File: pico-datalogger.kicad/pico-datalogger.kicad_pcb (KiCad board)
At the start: 2 copper layers, 21 x 33.8 mm, 18 parts, among them J1 JST-PH2 Bat, J2 Pico Pin 1-13, J3 Pico Pin 40-28, J4 Alt-Bat, SW1 SW_Push_SLIM, U1 SN74HC74N, U2 PCF8563T, Y1 Crystal

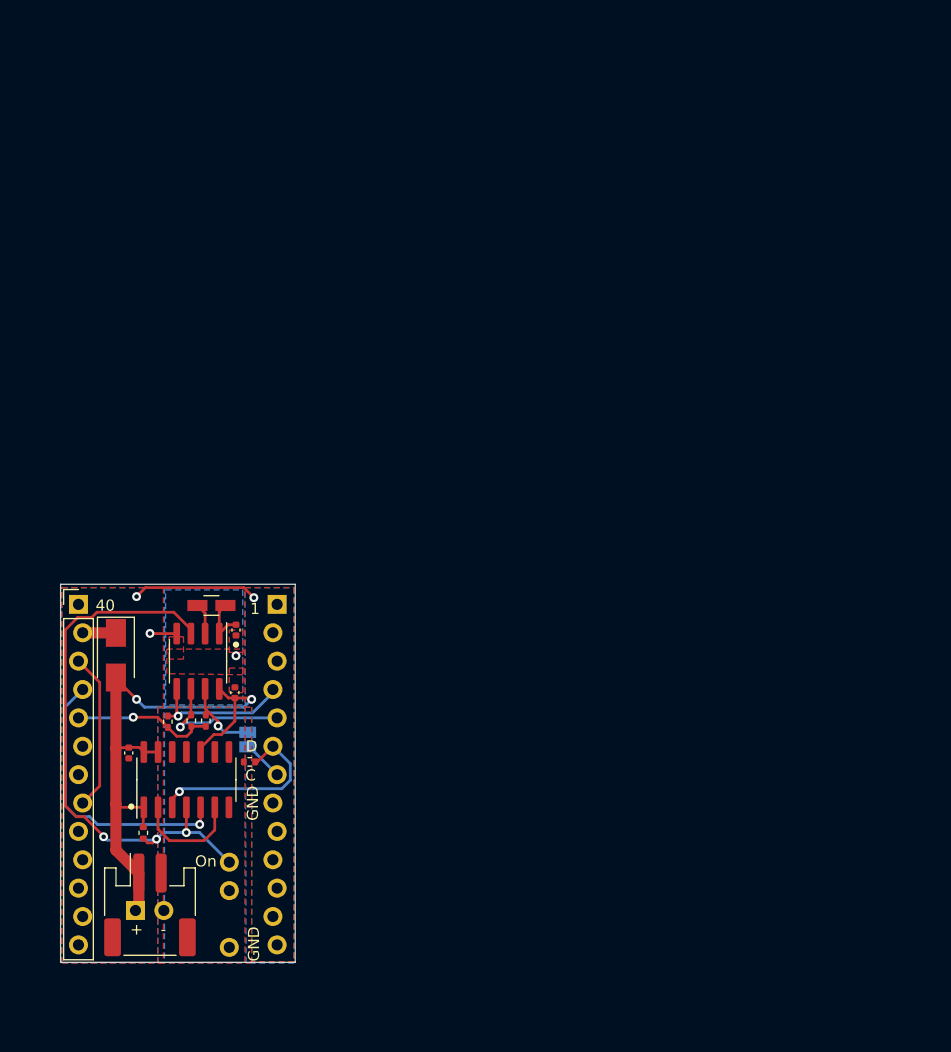
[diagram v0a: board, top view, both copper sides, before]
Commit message: Rev. 0.9: initial routing
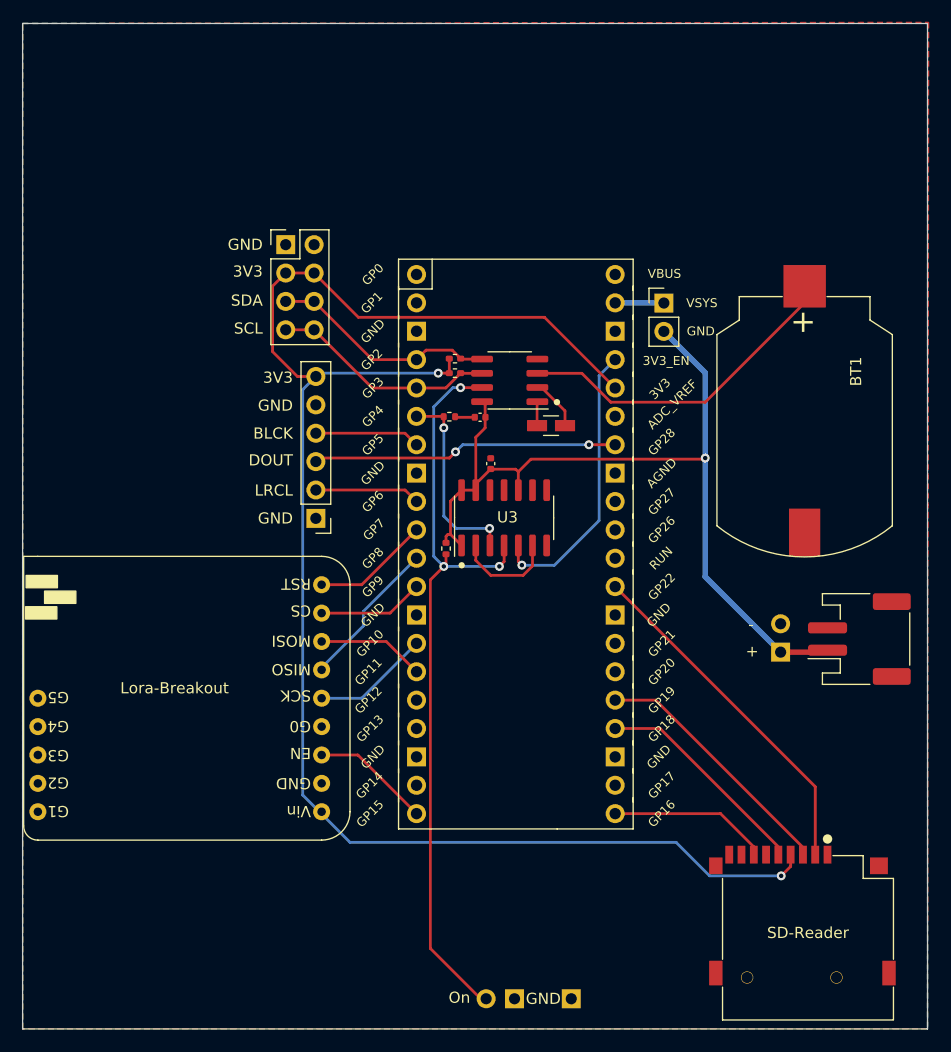
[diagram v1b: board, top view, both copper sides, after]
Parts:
- removed C3: 22pF, Capacitor_SMD:C_0402_1005Metric
- removed D1: D_Schottky, Diode_SMD:D_SMA
- removed R5: 10K, Resistor_SMD:R_0402_1005Metric
- added BT1: Coin_Cell, user:CR2032_Holder, F.Cu at (165.0, 82.5)
- added J5: Conn_I2S, Connector_PinHeader_2.54mm:PinHeader_1x06_P2.54mm_Vertical, F.Cu at (121.2, 92.3)
- added J7: Micro_SD_TF_PUSH, user:TF-Push, F.Cu at (164.8, 127.7)
- added U3: Pico, user:RPi_Pico_TH_nodbg, F.Cu at (139.2, 94.6)
- J1: value JST-PH2 Bat -> JST-PH2 VCC
- J2: value Pico Pin 1-13 -> Conn_I2C_Internal; footprint user:Connector_1x13_no_solder -> Connector_PinHeader_2.54mm:PinHeader_2x04_P2.54mm_Vertical; moved to F.Cu
- J3: value Pico Pin 40-28 -> RFM9x_Lora_Breakout; footprint user:Connector_1x13_no_solder -> user:RFM9x_Lora_Breakout
- J4: value Alt-Bat -> Alt-VCC
- JP1: value Jmp_CLKOUT -> Jumper_VSYS; footprint Jumper:SolderJumper-2_P1.3mm_Open_Pad1.0x1.5mm -> Connector_PinHeader_2.54mm:PinHeader_1x02_P2.54mm_Vertical; moved to F.Cu
- U2: value PCF8563T -> PCF8523T
- moved J1 67.8 mm to (169.9, 103.1), turned to 90 degrees
- moved J4 62.2 mm to (162.8, 104.3), turned to 0 degrees
- moved JP1 54.0 mm to (152.4, 73.0), turned to 0 degrees
- moved C1 41.5 mm to (136.9, 87.4), turned to 90 degrees
- moved R4 40.4 mm to (133.7, 79.3), turned to 0 degrees
- moved R3 40.1 mm to (133.7, 78.0), turned to 0 degrees
- moved U2 37.6 mm to (138.6, 80.0), turned to 180 degrees
- moved R2 37.2 mm to (132.9, 95.0)
- moved U1 36.9 mm to (138.1, 92.2)
- moved R1 35.7 mm to (133.2, 83.2), turned to 180 degrees
- moved Y1 34.4 mm to (142.3, 84.0), turned to 0 degrees
- moved C2 33.0 mm to (135.9, 83.2), turned to 180 degrees
- moved J2 32.2 mm to (118.5, 67.8), turned to 0 degrees
- moved SW1 31.0 mm to (144.1, 135.3), turned to 180 degrees
- moved J3 28.6 mm to (121.8, 118.6), turned to 90 degrees
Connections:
- J2 pad 1: unconnected-(J2-Pad1) -> GND
- J2 pad 2: unconnected-(J2-Pad2) -> GND
- J2 pad 3: GND -> +3V3
- J2 pad 4: /SDA -> +3V3
- J2 pad 5: /SCL -> /SDA
- J2 pad 6: /GP4_DONE -> /SDA
- J2 pad 7: /GP5_CLKOUT -> /SCL
- J2 pad 8: GND -> /SCL
- J3 pad 1: unconnected-(J3-Pad1) -> +3V3
- J3 pad 11: unconnected-(J3-Pad11) -> (no net)
- J3 pad 12: unconnected-(J3-Pad12) -> (no net)
- J3 pad 13: GND -> (no net)
- J3 pad 2: /VSYS -> GND
- J3 pad 3: GND -> /Lora_EN
- J3 pad 4: /3V3_EN -> unconnected-(J3-Pad4)
- J3 pad 5: +3V3 -> /SCLK1
- J3 pad 6: unconnected-(J3-Pad6) -> /MISO1
- J3 pad 7: unconnected-(J3-Pad7) -> /MOSI1
- J3 pad 8: GND -> /Lora_CS
- J3 pad 9: unconnected-(J3-Pad9) -> /Lora_RST
- JP1 pad 1: /GP5_CLKOUT -> /VSYS
- JP1 pad 2: /CLKOUT -> +BATT
- R3 pad 1: /SCL -> +3V3
- R3 pad 2: +3V3 -> /SDA
- R4 pad 1: /SDA -> +3V3
- R4 pad 2: +3V3 -> /SCL
- U2 pad 3: /1~{PRE} -> Net-(BT1-Pad1)
- U2 pad 7: /CLKOUT -> /1~{PRE}
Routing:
- net +3V3: track 12.8 -> 145.5 mm, vias 1 -> 2
- net /SD_CS: track 0.00 -> 31.4 mm
- net Net-(BT1-Pad1): track 0.00 -> 30.2 mm
- net /DOUT: track 0.00 -> 27.4 mm, vias 0 -> 2
- net GND: track 27.7 -> 1.78 mm, vias 4 -> 0
- net +BATT: track 53.6 -> 77.7 mm, vias 2 -> 1
- net /MOSI0: track 0.00 -> 22.9 mm
- net /SCLK0: track 0.00 -> 19.8 mm
- net /1~{PRE}: track 49.8 -> 69.5 mm
- net /MISO0: track 0.00 -> 14.3 mm
- net /MISO1: track 0.00 -> 13.6 mm
- net /Lora_EN: track 0.00 -> 10.9 mm
- net /SCLK1: track 0.00 -> 10.7 mm
- net /Lora_RST: track 0.00 -> 10.7 mm
- net /MOSI1: track 0.00 -> 9.82 mm
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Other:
- board size 21 x 33.8 mm -> 81 x 90 mm
- board text added: "3V3"
- board text added: "BLCK"
- board text added: "DOUT"
- board text added: "LRCL"
- board text added: "Lora-Breakout"
- board text added: "Pico Inky Pack"
- board text added: "SD-Reader"
- board text removed: "1"
- board text removed: "40"
- board text removed: "C"
- board text removed: "D"
- board text removed: "GP4_DONE"
- board text removed: "GP5_CLKOUT"
- board text removed: "github.com/bablokb/pico-en-control Rev. 3.1"
